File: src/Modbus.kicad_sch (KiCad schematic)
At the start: 7 parts, among them U2 SP3485

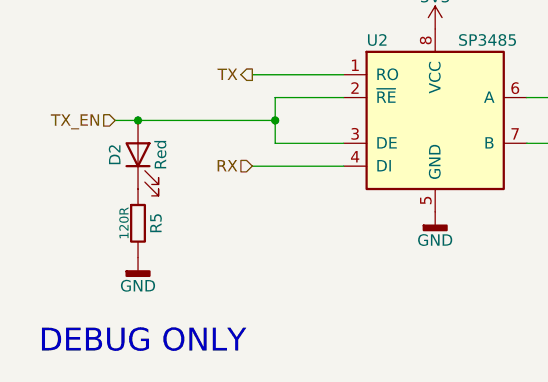
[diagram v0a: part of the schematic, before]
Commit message: ongoing work
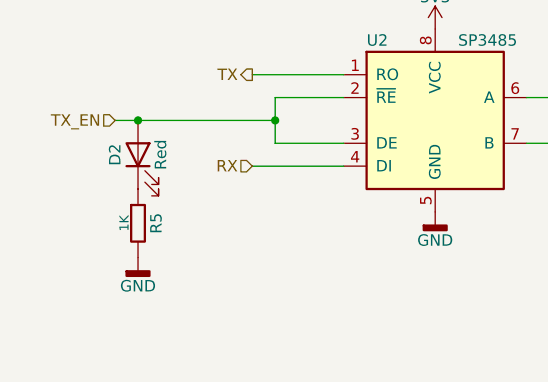
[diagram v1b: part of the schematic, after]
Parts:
- removed R5: 120R, 7Sigma:R_0402_1005Metric, symbol Resistor:0402WGF1200TCE
- added R5: 1K, 7Sigma:R_0402_1005Metric, symbol Resistor:0402WGF1001TCE
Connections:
- net GND: now also R5.2
- net at D2.1 (K): now also R5.1
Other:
- note removed: "DEBUG ONLY"

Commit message: Layout progress
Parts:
- C6: Price @1 USD (none) -> 0.0015; Price @100 USD (none) -> 0.0015; Price @Bulk USD (none) -> 0.0012; Price Bulk Qty (none) -> 1000; Price Source (none) -> LCSC; Price Updated (none) -> 2026-05-14
- D2: Price @1 USD (none) -> 0.0396; Price @100 USD (none) -> 0.0396; Price @Bulk USD (none) -> 0.0266; Price Bulk Qty (none) -> 600; Price Source (none) -> LCSC; Price Updated (none) -> 2026-05-14
- R1, R3, R4, R5: Price @1 USD (none) -> 0.0011; Price @100 USD (none) -> 0.0011; Price @Bulk USD (none) -> 0.0009; Price Bulk Qty (none) -> 1000; Price Source (none) -> LCSC; Price Updated (none) -> 2026-05-14
- U2: Price @1 USD (none) -> 0.3077; Price @100 USD (none) -> 0.2063; Price @Bulk USD (none) -> 0.1685; Price Bulk Qty (none) -> 1000; Price Source (none) -> LCSC; Price Updated (none) -> 2026-05-14
